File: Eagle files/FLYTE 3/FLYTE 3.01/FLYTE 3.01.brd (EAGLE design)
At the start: 83.7 x 65.7 mm, 307 parts, among them IC1 BMP280, IC2 MPXV5100DP, IC3 AS179-92LF, IC4 AS179-92LF, IC6 MAX8574EUT+T, IC8 MCP73843-420I_MS, IC9 MCP73844-840I_MS, J10 B2B-XH-A(LF)(SN), J11 B2B-XH-A(LF)(SN), J12 CON-SMA-EDGE-S, J13 282834-2, J2 282834-2, J3 282834-2, J4 282834-2, J5 282834-2, J6 503182-1852, J7 XT60-M, J8 CON-SMA-EDGE-S, J9 282834-2, Q1 SI7625DN-T1-GE3, Q6 SI7625DN-T1-GE3, Q7 SI7625DN-T1-GE3, U1 BNO055, U2 CJ3400, U3 CJ3400, U5 CJ3400, U6 ADS1115IDGSR, U7 CJ3400, U9 ADS1115IDGSR, X6 USB Type C, Y1 FC-135_32.7680KA-A0

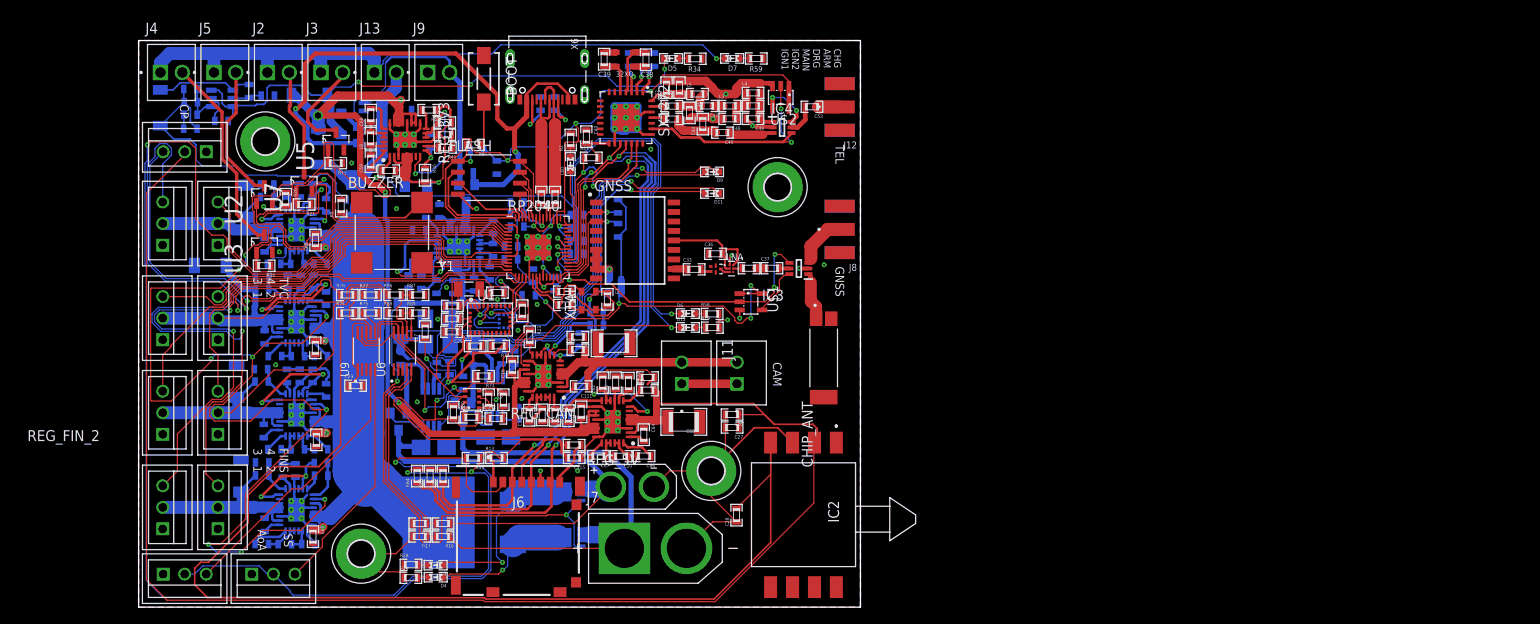
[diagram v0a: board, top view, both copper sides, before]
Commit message: FLYTE 3.02
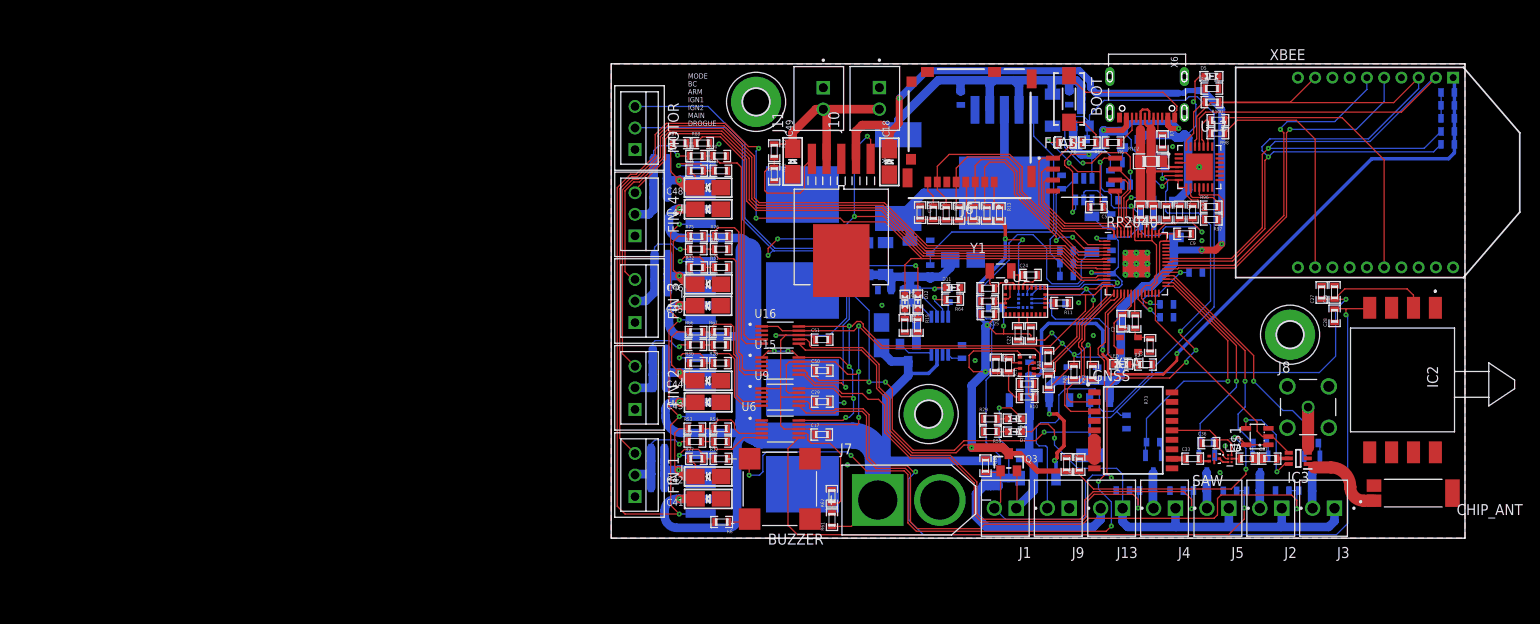
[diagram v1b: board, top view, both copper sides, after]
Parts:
- removed 1S_POW: V60D60C-M3_I, V60D60C-M3_I:V60D60CM3I
- removed 32XO: ASE, crystal:ASE
- removed AOA, SS, TVC_1, TVC_2, TVC_3, TVC_4: 03-JST-B3B-XH-A, bt_con-jst-xh (1):B3B-XH
- removed C102, C106, C68, C75, C82, C89: 10 uF, standardparts:0603
- removed C103, C109, C69, C76, C83, C90: 4.7 uF, standardparts:0603
- removed C104: 1.2 nF, standardparts:0603
- removed C105, C111, C64, C71, C78, C85, C92: 22 nF, standardparts:0603
- removed C107, C108, C113, C114, C66, C67, C73, C74, C80, C81, C87, C88, C94, C95: 0.22 uF, standardparts:0603
- removed C110, C70, C77, C84, C91: 1.8 nF, standardparts:0603
- removed C112: 100 uF, standardparts:1210
- removed C65: 220 uF, standardparts:1210
- removed C72, C79, C86, C93: 100 uF, standardparts:1206
- removed C96, C98: 10uF, microbuilder:EIA3216-18/A-W
- removed C97: 0.1 uF, standardparts:0603
- removed CHG_BST, REG_3V3, REG_5V, REG_CAM, REG_FIN_1, REG_FIN_2, REG_TVC_1, REG_TVC_2: LT3120JV#PBF, LT3120JV#PBF:QFN50P400X500X83-29N
- removed D3, D9: (no value), standardparts:0603.LED
- removed D8: RSX501LAM20TR, RSX501LAM20TR:SODFL4725X105N
- removed H1: MOUNT-PAD-ROUND3.0, holes:3,0-PAD
- removed IC4: AS179-92LF, AS179-92LF:SOT65P220X100-6N
- removed IC8: MCP73843-420I_MS, MCP73843-420I_MS:SOP65P490X110-8N
- removed J12: CON-SMA-EDGE-S, CON-SMA-EDGE-S:RFSOLUTIONS_CON-SMA-EDGE-S
- removed L10, L11, L12, L13, L14, L15, L16, L9: 4.7 uH, standardparts:0603
- removed L2: 2.7 nH, standardparts:0603
- removed L3, L4: 5.6 nH, standardparts:0603
- removed L5: 33 nH, standardparts:0603
- removed Q6, Q7: SI7625DN-T1-GE3, SI7625DN-T1-GE3:SIS862DNT1GE3
- removed SX1272: SX1272IMLTRT, SX1272IMLTRT:QFN65P600X600X100-29N
- removed U$11: XT30UPB-M, XT30UPB-M:XT30UPB-M
- removed U$2: SN74LVC1G04DBVR, SN74LVC1G04DBVR:SOT23-5
- added J1: 282834-2, 282834-2:TE_282834-2
- added R100, R98, R99: 0 ohm, standardparts:0603
- added R101, R93, R94, R95, R96: 10k ohm, standardparts:0603
- added R102: (no value), standardparts:0805
- added R12, R57, R71, R91: 100k ohm, standardparts:0603
- added R90, R92: 140k ohm, standardparts:0603
- added R97: (no value), standardparts:0603
- added U10, U4: LM1117-3.3, LM1117-3.3:SOT230
- added U11, U12, U13, U14, U8: MIC29302WU-TR, MIC29302WU:TO-263-5_MCH
- added U15, U16: ADS1115IDGSR, ADS1115IDGSR:SOP50P490X110-10N
- added U17: CP2102, CP2102:QFN50P500X500X100-29N
- added VR1: XL6009, XL6009:DPAK170P1435X465-6N
- added XBEE: XBP9B-XCST-021, XBP9B-XCST-021:DIP2200W51P200L3294H279Q20P
- C1: value 10 uF -> (none)
- C18: value 10 uF -> 10uF; device standardparts:0603 -> microbuilder:EIA3216-18/A-W
- C34: value 3.3 nF -> 47pF
- C35: value 22 nF -> (none)
- C38: value 24 pF -> (none)
- C39: value 24 pF -> 1uF
- C4: value 4.7 uF -> (none)
- C40: value 100 nF -> 10uF
- C41, C43: value 100 nF -> 10uF; device standardparts:0603 -> microbuilder:EIA3216-18/A-W
- C42: value 100 nF -> 10 uF; device standardparts:0603 -> microbuilder:EIA3216-18/A-W
- C44, C49: value 3.3 pF -> 10 uF; device standardparts:0603 -> microbuilder:EIA3216-18/A-W
- C45: value 47 pF -> 10uF; device standardparts:0603 -> microbuilder:EIA3216-18/A-W
- C46, C48: value 8.2 pF -> 10 uF; device standardparts:0603 -> microbuilder:EIA3216-18/A-W
- C47: value 22 pF -> 10uF; device standardparts:0603 -> microbuilder:EIA3216-18/A-W
- C50: value 1.5 pF -> 0.1 uF
- C51: value 10 nF -> 0.1 uF
- C52: value 47 pF -> 100 uF; device standardparts:0603 -> standardparts:1206
- C53: value 47 pF -> 1 uF
- C58: device standardparts:0805 -> standardparts:1206
- C59: value 0.22 uF -> 1 uF
- C60: value 0.22 uF -> 100 uF; device standardparts:0603 -> standardparts:1206
- C61: value 10 uF -> 100 nF
- C63: value 1.8 nF -> 1 uF
- J8: value CON-SMA-EDGE-S -> SMA_CONNECTOR; device CON-SMA-EDGE-S:RFSOLUTIONS_CON-SMA-EDGE-S -> SMA_CONNECTOR (1):LPRS_SMA_CONNECTOR
- L1: value 10 nH -> 33 uH; device standardparts:0603 -> SRR1260-330M:INDP125125X600N
- R16: value 412k ohm -> 365k ohm
- R17: value 100k ohm -> 57.6k ohm
- R18: value 137k ohm -> 100k ohm
- R22, R53: value 46.4k ohm -> 100k ohm
- R23: value 158k ohm -> 301k ohm
- R24: value 523k ohm -> 0.1 ohm
- R25, R37: value 100k ohm -> 0.13 ohm
- R27: value 10k ohm -> 301k ohm
- R28: value 105 ohm -> 100k ohm
- R30: value 316k ohm -> 301k ohm
- R32: value 46.4k ohm -> 301k ohm
- R33: value 158k ohm -> 100k ohm
- R35: value 523k ohm -> 301k ohm
- R38, R45, R49: value 46.4k ohm -> 0.13 ohm
- R39, R42, R46, R50: value 158k ohm -> 0.13 ohm
- R40, R47, R51: value 402k ohm -> 0.13 ohm
- R41: value 21k ohm -> 0.13 ohm
- R44, R48, R52: value 50k ohm -> 0.13 ohm
- R54, R67, R86, R88: value 158k ohm -> 140k ohm
- R55: value 402k ohm -> 100k ohm
- R56: value 50k ohm -> 140k ohm
- R60: value 0.1 ohm -> 140k ohm
- R61: value 158 ohm -> 100k ohm
- R62, R69: value 100k ohm -> 140k ohm
- R68: value 1.3M ohm -> 100k ohm
- R74: value 36.5k ohm -> 140k ohm
- R76: value 43k ohm -> 140k ohm
- R78: value 28k ohm -> 140k ohm
- moved J4 125.8 mm to (126.2, 48.5), turned to 180 degrees
- moved J5 125.7 mm to (132.3, 48.5), turned to 180 degrees
- moved J2 125.7 mm to (138.5, 48.5), turned to 180 degrees
- moved J3 125.6 mm to (144.6, 48.5), turned to 180 degrees
- moved H4 120.9 mm to (140.7, 68.6)
- moved U5 119.2 mm to (143.3, 53.5), flipped to the bottom, turned to 270 degrees
- moved R15 117.7 mm to (143.2, 56.0), flipped to the bottom, turned to 0 degrees
- moved C34 116.4 mm to (159.0, 96.7), flipped to the bottom, turned to 180 degrees
- moved U7 115.6 mm to (137.3, 53.5), flipped to the bottom, turned to 270 degrees
- moved R21 114.2 mm to (137.2, 56.0), flipped to the bottom, turned to 0 degrees
- moved U2 113.7 mm to (131.1, 53.6), flipped to the bottom, turned to 270 degrees
- moved R26 110.5 mm to (131.1, 56.1), flipped to the bottom, turned to 0 degrees
- moved R74 110.3 mm to (139.8, 50.5), flipped to the bottom
- moved D1 109.0 mm to (117.7, 80.2)
- moved U3 106.2 mm to (124.9, 53.6), flipped to the bottom, turned to 270 degrees
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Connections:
- removed net 1S_ADC: R78.2, R79.1, U6.5
- removed net 1S_POW: 1S_POW.1, D3.P$1, Q7.10, Q7.11, Q7.5, Q7.6, Q7.7, Q7.8, Q7.9
- removed net 2S_ADC: R16.2, R17.1, U6.4
- removed net 2S_POW: 1S_POW.2, D4.P$1, Q6.10, Q6.11, Q6.5, Q6.6, Q6.7, Q6.8, Q6.9
- removed net ADC_AVDD: RP2040.43
- removed net AIN2: R88.2, R89.1, U6.6
- removed net AIN3: R86.2, R87.1, U6.7
- removed net AOA_ADC: AOA.P$3, U9.4
- removed net CS_SX: R27.1, RP2040.32, SX1272.20
- removed net F1: R30.1, R31.2, REG_3V3.9
- removed net F2: R35.1, R37.2, REG_5V.9
- removed net F3: R40.1, R44.2, REG_FIN_1.9
- removed net F4: R47.1, R48.2, REG_FIN_2.9
- removed net F5: R51.1, R52.2, REG_TVC_1.9
- removed net F6: R55.1, R56.2, REG_TVC_2.9
- removed net F7: CHG_BST.9, R68.1, R69.2
- removed net F8: R24.1, R25.2, REG_CAM.9
- removed net N$100: IC8.1, Q3.2, R60.2
- removed net N$101: D9.P$2, R61.1
- removed net N$102: IC8.3, R61.2
- removed net N$103: IC8.4, R62.1
- removed net N$104: IC8.8, Q3.1
- removed net N$106: C97.2, IC8.5
- removed net N$111: CHG_BST.10, R66.2
- removed net N$112: C104.2, R66.1
- removed net N$113: CHG_BST.14, R67.2
- removed net N$114: C105.2, CHG_BST.1
- removed net N$115: C107.2, CHG_BST.26, CHG_BST.27, L15.1
- removed net N$116: C108.1, CHG_BST.24, CHG_BST.25, L15.2
- removed net N$117: C107.1, CHG_BST.28
- removed net N$118: C108.2, CHG_BST.23
- removed net N$119: R23.2, REG_CAM.14
- removed net N$120: C111.2, REG_CAM.1
- removed net N$122: C113.2, L16.1, REG_CAM.26, REG_CAM.27
- removed net N$123: C114.1, L16.2, REG_CAM.24, REG_CAM.25
- removed net N$124: C113.1, REG_CAM.28
- removed net N$125: C114.2, REG_CAM.23
- removed net N$46: R42.2, REG_3V3.14
- removed net N$47: C35.2, REG_3V3.1
- removed net N$48: C60.1, L9.2, REG_3V3.24, REG_3V3.25
- removed net N$49: C59.1, REG_3V3.28
- removed net N$52: D3.P$2, R28.2
- removed net N$56: C60.2, REG_3V3.23
- removed net N$57: R32.2, REG_5V.10
- removed net N$58: C63.2, R32.1
- removed net N$59: R33.2, REG_5V.14
- removed net N$60: C64.2, REG_5V.1
- removed net N$61: C66.2, L10.1, REG_5V.26, REG_5V.27
- removed net N$62: C67.1, L10.2, REG_5V.24, REG_5V.25
- removed net N$63: C66.1, REG_5V.28
- removed net N$64: C67.2, REG_5V.23
- removed net N$65: R38.2, REG_FIN_1.10
- removed net N$66: C70.2, R38.1
- removed net N$67: R39.2, REG_FIN_1.14
- removed net N$68: C71.2, REG_FIN_1.1
- removed net N$69: C73.2, L11.1, REG_FIN_1.26, REG_FIN_1.27
- removed net N$70: C74.1, L11.2, REG_FIN_1.24, REG_FIN_1.25
- removed net N$71: C73.1, REG_FIN_1.28
- removed net N$72: C74.2, REG_FIN_1.23
- removed net N$73: R45.2, REG_FIN_2.10
- removed net N$74: C77.2, R45.1
- removed net N$75: R46.2, REG_FIN_2.14
- removed net N$76: C78.2, REG_FIN_2.1
- removed net N$77: C80.2, L12.1, REG_FIN_2.26, REG_FIN_2.27
- removed net N$78: C81.1, L12.2, REG_FIN_2.24, REG_FIN_2.25
- removed net N$79: C80.1, REG_FIN_2.28
- removed net N$80: C81.2, REG_FIN_2.23
- removed net N$81: R49.2, REG_TVC_1.10
- removed net N$82: C84.2, R49.1
- removed net N$83: R50.2, REG_TVC_1.14
- removed net N$84: C85.2, REG_TVC_1.1
- removed net N$85: C87.2, L13.1, REG_TVC_1.26, REG_TVC_1.27
- removed net N$86: C88.1, L13.2, REG_TVC_1.24, REG_TVC_1.25
- removed net N$87: C87.1, REG_TVC_1.28
- removed net N$88: C88.2, REG_TVC_1.23
- removed net N$89: R53.2, REG_TVC_2.10
- removed net N$90: C91.2, R53.1
- removed net N$91: R54.2, REG_TVC_2.14
- removed net N$92: C92.2, REG_TVC_2.1
- removed net N$93: C94.2, L14.1, REG_TVC_2.26, REG_TVC_2.27
- removed net N$94: C95.1, L14.2, REG_TVC_2.24, REG_TVC_2.25
- removed net N$95: C94.1, REG_TVC_2.28
- removed net N$96: C95.2, REG_TVC_2.23
- removed net N$99: C96.+, D8.1, D9.P$1, IC8.2, R60.1, R62.2
- removed net N_RXTX: IC4.6, U$2.4
- removed net P1: C4.1, REG_3V3.12, REG_3V3.13, REG_3V3.8
- removed net P2: C62.1, REG_5V.12, REG_5V.13, REG_5V.8
- removed net P3: C69.1, REG_FIN_1.12, REG_FIN_1.13, REG_FIN_1.8
- removed net P4: C76.1, REG_FIN_2.12, REG_FIN_2.13, REG_FIN_2.8
- removed net P5: C83.1, REG_TVC_1.12, REG_TVC_1.13, REG_TVC_1.8
- removed net P6: C90.1, REG_TVC_2.12, REG_TVC_2.13, REG_TVC_2.8
- removed net P7: C103.1, CHG_BST.12, CHG_BST.13, CHG_BST.8
- removed net P8: C109.1, REG_CAM.12, REG_CAM.13, REG_CAM.8
- removed net RXTX: IC4.4, SX1272.23, U$2.2
- removed net SS_ADC: SS.P$3, U9.5
- removed net TVC_1: RP2040.9, TVC_1.P$3
- removed net TVC_2: RP2040.8, TVC_2.P$3
- removed net TVC_3: RP2040.16, TVC_3.P$3
- removed net TVC_4: RP2040.6, TVC_4.P$3
- removed net VCC_CTRL: 1S_POW.3, C68.1, C75.1, C82.1, C89.1, Q1.1, Q1.2, Q1.3, REG_FIN_1.17, REG_FIN_1.19, REG_FIN_1.20, REG_FIN_1.21, REG_FIN_2.17, REG_FIN_2.19, REG_FIN_2.20, REG_FIN_2.21, REG_TVC_1.17, REG_TVC_1.19, REG_TVC_1.20, REG_TVC_1.21, REG_TVC_2.17, REG_TVC_2.19, REG_TVC_2.20, REG_TVC_2.21
- removed net V_TVC_1: C85.1, C86.2, R51.2, R86.1, REG_TVC_1.2, REG_TVC_1.4, REG_TVC_1.5, REG_TVC_1.6, TVC_1.P$2, TVC_2.P$2
- removed net V_TVC_2: C92.1, C93.2, R55.2, REG_TVC_2.2, REG_TVC_2.4, REG_TVC_2.5, REG_TVC_2.6, TVC_3.P$2, TVC_4.P$2
- removed net XIN1: 32XO.3, C38.2, SX1272.4
- removed net XOUT1: 32XO.1, C39.2, SX1272.5
- removed net XT30+: C98.+, IC8.7, Q3.3, Q7.1, Q7.2, Q7.3, R78.1, U$11.P$1
- new net 3V3_OP: AC1.1, AC1.10, AC1.3, AC1.7, C10.2, C11.2, C115.2, C12.2, C13.2, C14.2, C15.2, C16.2, C19.2, C20.1, C21.1, C25.1, C30.2, C31.2, C32.2, C5.1, C61.2, C9.2, FLASH.8, IC1.6, IC1.8, J6.4, L6.1, Q3.3, R0.2, R10.2, R13.2, R14.1, R43.1, R72.2, R73.2, R80.2, R81.2, R82.2, R83.2, R84.2, R85.2, RP2040.1, RP2040.10, RP2040.22, RP2040.26, RP2040.33, RP2040.42, RP2040.43, RP2040.44, RP2040.48, RP2040.49, U$1.1, U$1.5, U1.28, U1.3, U1.4, U16.7
- new net 3V3_SET: C62.1, J1.2, Q3.1, R101.2, U17.6
- new net CTS: R98.1, XBEE.12
- new net D+1: R102.2, U17.4
- new net D1: FIN_1.P$2, R25.2, R37.2, R38.2, R39.2, R55.1
- new net D2: FIN_2.P$2, R45.2, R46.2, R47.2, R48.2, R68.1
- new net D3: FIN_3.P$2, R40.2, R41.2, R42.2, R44.2, R77.1
- new net D4: FIN_4.P$2, R49.2, R50.2, R51.2, R52.2, R89.1
- new net DTR: R100.1, XBEE.9
- new net N$13: R28.1, R30.2, U11.5
- new net N$18: D10.2, L1.1, VR1.3, VR1.6
- new net N$20: R55.2, R56.1, U6.5
- new net N$5: R12.1, R27.2, U8.5
- new net RSSI: RP2040.35, XBEE.6
- new net RTS: R99.1, XBEE.16
- new net TEL_RST: RP2040.34, XBEE.5
- new net TEL_RX: R93.1, RP2040.36, U17.26, XBEE.3
- new net TEL_TX: R94.1, RP2040.37, U17.25, XBEE.2
- new net V_FIN_3: C46.+, R32.1, R40.1, R41.1, R42.1, R44.1, R75.1, U12.4
- new net V_FIN_4: C48.+, R35.1, R49.1, R50.1, R51.1, R52.1, R87.1, U13.4
- net 3V3: now also C34.2, C39.2, C4.2, J1.1, Q3.2, R93.2, R94.2, U4.2, U4.4, XBEE.1; no longer AC1.1, AC1.10, AC1.3, AC1.7, AOA.P$2, C10.2, C11.2, C115.2, C12.2, C13.2, C14.2, C15.2, C16.2, C17.1, C19.2, C20.1, C21.1, C25.1, C29.1, C30.2, C31.2, C32.2, C35.1, C41.2, C5.1, C58.2, C9.2, FLASH.8, IC1.6, IC1.8, J6.4, L6.1, R0.2, R10.2, R13.2, R14.1, R27.2, R30.2, R43.1, R72.2, R73.2, R80.2, R81.2, R82.2, R83.2, R84.2, R85.2, REG_3V3.2, REG_3V3.4, REG_3V3.5, REG_3V3.6, RP2040.1, RP2040.10, RP2040.22, RP2040.26, RP2040.33, RP2040.42, RP2040.44, RP2040.48, RP2040.49, SS.P$2, SX1272.1, SX1272.15, U$1.1, U$1.5, U$2.1, U$2.5, U1.28, U1.3, U1.4, U6.8, U9.1, U9.8
- net 5V: now also C17.1, C29.1, C38.2, C50.1, C51.1, U10.2, U10.4, U15.8, U16.8, U6.8, U9.1, U9.8; no longer C64.1, C65.2, R35.2, REG_5V.2, REG_5V.4, REG_5V.5, REG_5V.6
- net BUZZER: now also RP2040.17; no longer RP2040.14
- net CAM: now also RP2040.11, U14.1; no longer REG_CAM.16, RP2040.35
- net CS_SD: now also RP2040.3; no longer RP2040.7
- net CTRL: now also RP2040.12, U11.1, U12.1, U13.1, U8.1; no longer REG_FIN_1.16, REG_FIN_2.16, REG_TVC_1.16, REG_TVC_2.16, RP2040.36
- net D+: now also R102.1
- net D-: now also U17.5
- net DROGUE: now also RP2040.32; no longer RP2040.2
- net FIN_1: now also RP2040.6; no longer RP2040.13
- net FIN_2: now also RP2040.7; no longer RP2040.15
- net FIN_3: now also RP2040.8; no longer RP2040.11
- net FIN_4: now also RP2040.9; no longer RP2040.12
- net GND: now also C1.1, C18.-, C35.1, C4.1, C41.-, C42.-, C43.-, C44.-, C45.-, C46.-, C47.-, C48.-, C49.-, C50.2, C52.1, C53.1, C59.1, C60.1, C61.1, C63.2, R101.1, R12.2, R22.2, R28.2, R31.2, R33.2, R54.2, R56.2, R60.2, R62.2, R67.2, R69.2, R74.2, R76.2, R78.2, R86.2, R88.2, R90.2, R92.2, R95.1, R97.2, U10.1, U11.3, U11.6, U12.3, U12.6, U13.3, U13.6, U14.3, U14.6, U15.3, U16.3, U17.29, U17.3, U17.P$1, U4.1, U8.3, U8.6, VR1.1, XBEE.10; no longer 32XO.2, 32XO.4, AOA.P$1, C1.2, C102.2, C103.2, C104.1, C106.1, C109.2, C110.1, C112.1, C18.2, C4.2, C41.1, C42.1, C43.1, C44.2, C46.2, C48.2, C49.2, C52.2, C61.2, C63.1, C65.1, C68.2, C69.2, C70.1, C72.1, C75.2, C76.2, C77.1, C79.1, C82.2, C83.2, C84.1, C86.1, C89.2, C90.2, C91.1, C93.1, C96.-, C97.1, C98.-, CHG_BST.11, CHG_BST.15, CHG_BST.18, CHG_BST.22, CHG_BST.29, CHG_BST.3, CHG_BST.P$1, CHG_BST.P$2, CHG_BST.P$3, CHG_BST.P$4, CHG_BST.P$5, CHG_BST.P$6, H1.B3,0, IC4.2, IC8.6, J12.G1, J12.G2, J12.G3, J12.G4, R23.1, R25.1, R28.1, R31.1, R33.1, R37.1, R39.1, R42.1, R44.1, R46.1, R48.1, R50.1, R52.1, R54.1, R56.1, R67.1, R69.1, R75.2, R77.2, R79.2, R87.2, R89.2, REG_3V3.11, REG_3V3.15, REG_3V3.18, REG_3V3.22, REG_3V3.29, REG_3V3.3, REG_3V3.P$1, REG_3V3.P$2, REG_3V3.P$3, REG_3V3.P$4, REG_3V3.P$5, REG_3V3.P$6, REG_5V.11, REG_5V.15, REG_5V.18, REG_5V.22, REG_5V.29, REG_5V.3, REG_5V.P$1, REG_5V.P$2, REG_5V.P$3, REG_5V.P$4, REG_5V.P$5, REG_5V.P$6, REG_CAM.11, REG_CAM.15, REG_CAM.18, REG_CAM.22, REG_CAM.29, REG_CAM.3, REG_CAM.P$1, REG_CAM.P$2, REG_CAM.P$3, REG_CAM.P$4, REG_CAM.P$5, REG_CAM.P$6, REG_FIN_1.11, REG_FIN_1.15, REG_FIN_1.18, REG_FIN_1.22, REG_FIN_1.29, REG_FIN_1.3, REG_FIN_1.P$1, REG_FIN_1.P$2, REG_FIN_1.P$3, REG_FIN_1.P$4, REG_FIN_1.P$5, REG_FIN_1.P$6, REG_FIN_2.11, REG_FIN_2.15, REG_FIN_2.18, REG_FIN_2.22, REG_FIN_2.29, REG_FIN_2.3, REG_FIN_2.P$1, REG_FIN_2.P$2, REG_FIN_2.P$3, REG_FIN_2.P$4, REG_FIN_2.P$5, REG_FIN_2.P$6, REG_TVC_1.11, REG_TVC_1.15, REG_TVC_1.18, REG_TVC_1.22, REG_TVC_1.29, REG_TVC_1.3, REG_TVC_1.P$1, REG_TVC_1.P$2, REG_TVC_1.P$3, REG_TVC_1.P$4, REG_TVC_1.P$5, REG_TVC_1.P$6, REG_TVC_2.11, REG_TVC_2.15, REG_TVC_2.18, REG_TVC_2.22, REG_TVC_2.29, REG_TVC_2.3, REG_TVC_2.P$1, REG_TVC_2.P$2, REG_TVC_2.P$3, REG_TVC_2.P$4, REG_TVC_2.P$5, REG_TVC_2.P$6, SS.P$1, SX1272.16, SX1272.22, SX1272.26, SX1272.29, SX1272.P$1, SX1272.P$2, SX1272.P$3, SX1272.P$4, SX1272.P$5, SX1272.P$6, SX1272.P$7, SX1272.P$8, SX1272.P$9, TVC_1.P$1, TVC_2.P$1, TVC_3.P$1, TVC_4.P$1, U$11.P$2, U$2.3
- net GPS_RX: now also RP2040.15; no longer RP2040.27
- net GPS_TX: now also RP2040.16; no longer RP2040.28
- net IGN1: now also RP2040.29; no longer RP2040.5
- net IGN2: now also RP2040.30; no longer RP2040.4
- net LED: now also RP2040.18; no longer RP2040.37
- net MAIN: now also RP2040.31; no longer RP2040.3
- net MISO: now also RP2040.2; no longer RP2040.31, SX1272.18
- net MOS: now also D4.P$1
- net MOSI: now also RP2040.5; no longer RP2040.30, SX1272.19
- net N$14: now also R31.1, R32.2, U12.5; no longer R74.2, R75.1, U9.6
- net N$16: now also R22.1, R23.2, U14.5; no longer R22.2, REG_CAM.10
- net N$17: now also R33.1, R35.2, U13.5; no longer R76.2, R77.1, U9.7
- net N$19: now also R16.2, R17.1, VR1.5; no longer C110.2, R22.1
- net N$21: now also R53.2, R54.1, U6.4; no longer C59.2, L9.1, REG_3V3.26, REG_3V3.27
- net N$29: now also R57.2, R60.1, U6.6; no longer C42.2, SX1272.2
- net N$30: now also R61.2, R62.1, U6.7; no longer C43.2, SX1272.3
- net N$31: now also R66.2, R67.1, U9.4; no longer C44.1, C45.2, L1.2
- net N$32: now also R68.2, R69.1, U9.5; no longer C45.1, IC4.3
- net N$33: now also R71.2, R74.1, U9.6; no longer L2.1, SX1272.27
- net N$34: now also R75.2, R76.1, U15.4; no longer L1.1, SX1272.25
- net N$35: now also R77.2, R78.1, U15.5; no longer C46.1, C47.2, L2.2, L5.2
- net N$36: now also R79.2, R86.1, U15.6; no longer C47.1, L3.1
- net N$37: now also R87.2, R88.1, U16.4; no longer C48.1, C50.2, L3.2, L4.1
- net N$38: now also R89.2, R90.1, U16.5; no longer C49.1, C50.1, IC4.1, L4.2
- net N$39: now also R91.2, R92.1, U16.6; no longer C51.1, C52.1, L5.1, SX1272.28
- net N$40: now also R96.2, U17.9; no longer C53.2, IC4.5
- net N$41: now also R97.1, U17.11; no longer C53.1, J12.1
- net N$42: now also R98.2, U17.23; no longer C99.+, D10.1, D11.P$1, IC9.2, R63.1, R65.2
- net N$43: now also R99.2, U17.24; no longer R41.2, REG_3V3.10
- net N$44: now also R24.1
- net N$45: now also R100.2, U17.28; no longer C34.2, R41.1
- net PYRO_DROGUE: now also R71.1
- net PYRO_IGN1: now also R79.1
- net PYRO_IGN2: now also R91.1
- net PYRO_MAIN: now also R57.1
- net S: now also RP2040.27; no longer RP2040.34
- net SCK: now also RP2040.4; no longer RP2040.29, SX1272.17
- net SCL: now also RP2040.14, U15.1, U15.10, U16.10; no longer RP2040.18
- net SDA: now also RP2040.13, U15.9, U16.1, U16.9; no longer RP2040.17
- net USB+: now also C56.1, IC6.3, IC6.6
- net USB_BST: now also C58.2, C59.2, C60.2, C99.+, D10.1, D11.P$1, IC9.2, R16.1, R24.2, R63.1, R65.2; no longer C105.1, C106.2, CHG_BST.2, CHG_BST.4, CHG_BST.5, CHG_BST.6, D10.2, D8.2, Q6.4, Q7.4, R68.2
- net USB_CHG: now also C52.2, C53.2, L1.2, R95.2, VR1.2, VR1.4; no longer C102.1, CHG_BST.16, CHG_BST.17, CHG_BST.19, CHG_BST.20, CHG_BST.21
- net VBUS: now also C63.1, R96.1, U17.7, U17.8; no longer C56.1, IC6.3, IC6.6
- net VCC: now also C1.2, C18.+, C35.2, U10.3, U14.2, U4.3; no longer C1.1, C18.1, C61.1, REG_3V3.16, REG_3V3.17, REG_3V3.19, REG_3V3.20, REG_3V3.21, REG_5V.16, REG_5V.17, REG_5V.19, REG_5V.20, REG_5V.21, REG_CAM.17, REG_CAM.19, REG_CAM.20, REG_CAM.21
- net VOLT_DP: now also U9.7; no longer R74.1
- net VOLT_MOTOR: now also U15.7; no longer R76.1
- net V_CAM: now also C49.+, R23.1, U14.4; no longer C111.1, C112.2, R24.2, REG_CAM.2, REG_CAM.4, REG_CAM.5, REG_CAM.6
- net V_FIN_1: now also C42.+, R25.1, R27.1, R37.1, R38.1, R39.1, R53.1, U8.4; no longer C71.1, C72.2, FIN_1.P$2, FIN_2.P$2, R40.2, REG_FIN_1.2, REG_FIN_1.4, REG_FIN_1.5, REG_FIN_1.6
- net V_FIN_2: now also C44.+, R30.1, R45.1, R46.1, R47.1, R48.1, R66.1, U11.4; no longer C78.1, C79.2, FIN_3.P$2, FIN_4.P$2, R47.2, R88.1, REG_FIN_2.2, REG_FIN_2.4, REG_FIN_2.5, REG_FIN_2.6
- net XT60+: now also C41.+, C43.+, C45.+, C47.+, Q1.1, Q1.2, Q1.3, R61.1, U11.2, U12.2, U13.2, U8.2; no longer Q6.1, Q6.2, Q6.3, R16.1
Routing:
- net 3V3: track 409.6 -> 102.3 mm, vias 20 -> 2
- net 3V3_OP: track 0.00 -> 304.3 mm, vias 0 -> 21
- net GND: track 287.6 -> 37.2 mm, vias 30 -> 12
- net CS_SD: track 189.4 -> 25.3 mm
- net VCC_CTRL: track 102.9 -> 0.00 mm, vias 4 -> 0
- net XT60+: track 69.6 -> 169.1 mm, vias 0 -> 4
- net TEL_TX: track 0.00 -> 98.5 mm, vias 0 -> 1
- net TEL_RX: track 0.00 -> 97.1 mm, vias 0 -> 1
- net 3V3_SET: track 0.00 -> 78.4 mm, vias 0 -> 5
- net CTRL: track 247.9 -> 170.5 mm, vias 13 -> 6
- net N$33: track 1.58 -> 77.3 mm, vias 0 -> 1
- net BC: track 29.0 -> 102.5 mm, vias 0 -> 2
- net BUZZER: track 10.3 -> 82.9 mm, vias 0 -> 4
- net TVC_3: track 72.4 -> 0.00 mm, vias 1 -> 0
- net N$99: track 68.7 -> 0.00 mm, vias 1 -> 0
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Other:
- board size 83.7 x 65.7 mm -> 99 x 55 mm
- board text added: "MODE BC ARM IGN1 IGN2 MAIN DROGUE"
- board text removed: "CAM"
- board text removed: "CHG ARM DRG MAIN IGN2 IGN1"
- board text removed: "CP"
- board text removed: "FINS 4 2 3 1"
- board text removed: "GNSS"
- board text removed: "SS AoA"
- board text removed: "TEL"
- board text removed: "TVC 4 2 3 1"
